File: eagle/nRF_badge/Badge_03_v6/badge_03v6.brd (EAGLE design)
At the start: 30 x 70 mm, 43 parts, among them U1 LIS2DH12", U2 LP2985LV, U3 MCP6231, U5 M95M02, Y1 32768Hz

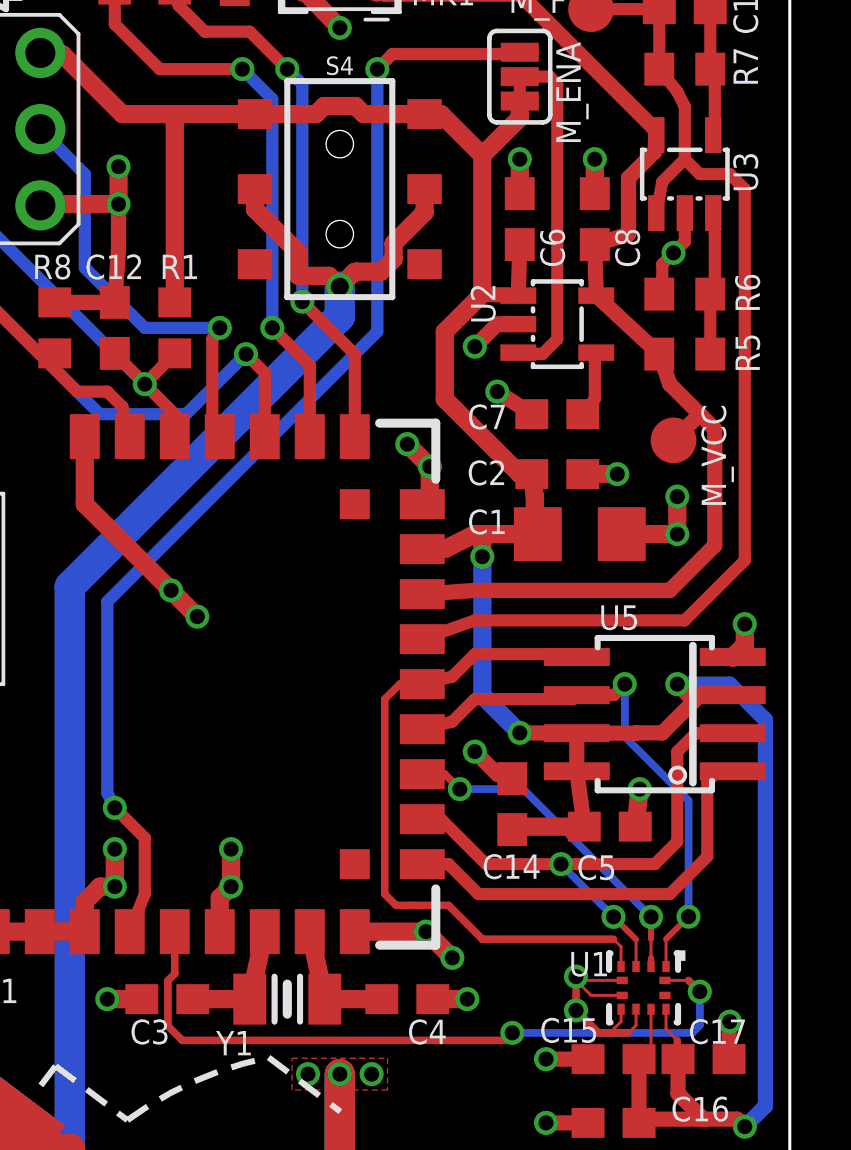
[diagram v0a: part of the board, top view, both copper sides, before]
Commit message: Updated DRC. Small fixed to board design
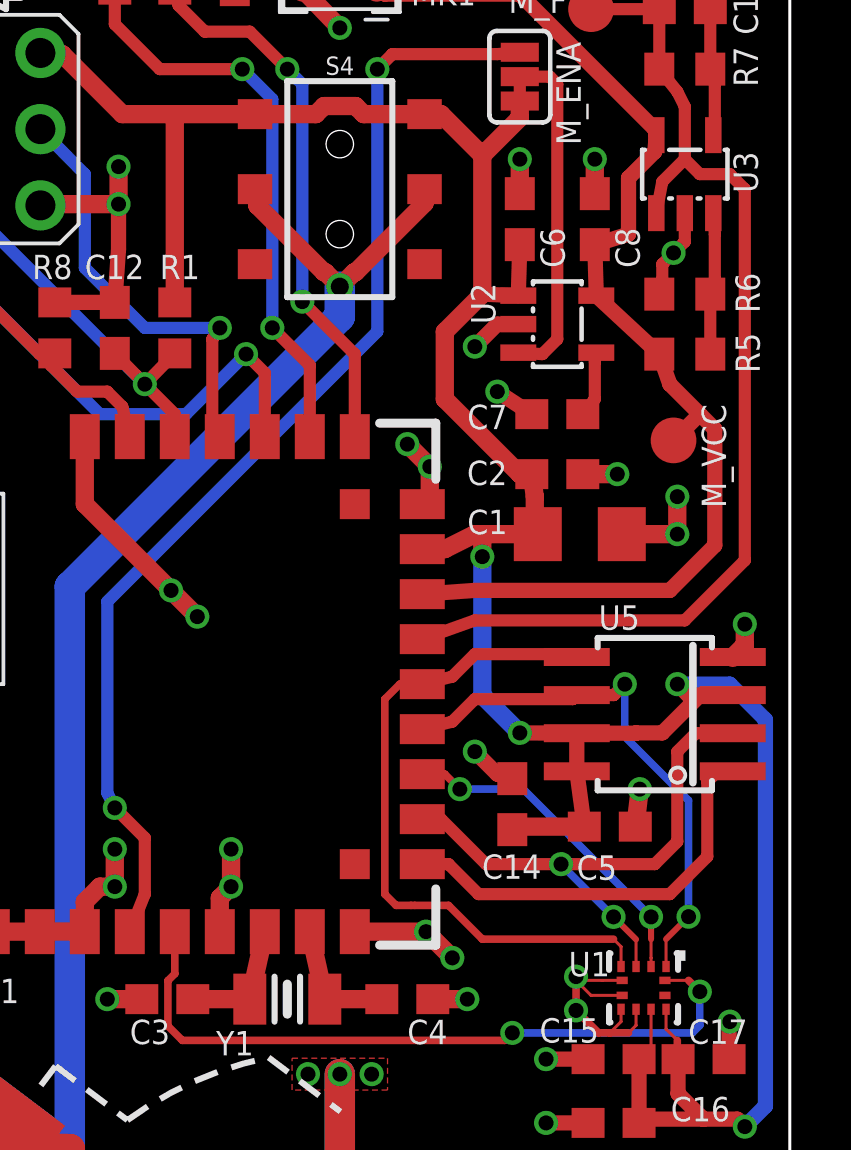
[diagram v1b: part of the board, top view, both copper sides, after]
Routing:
- net VBATT: track 140.7 -> 139.6 mm
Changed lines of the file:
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@@
 </class>
 </classes>
-<designrules name="PCBNG_DRC_by_oren *">
+<designrules name="PCBNG_DRC_by_oren">
 <description language="de">&lt;b&gt;EAGLE Design Rules&lt;/b&gt;
 &lt;p&gt;
@@
 <contactref element="S4" pad="5"/>
 <wire x1="12.25" y1="53" x2="12.175" y2="53" width="0.6096" layer="1"/>
-<wire x1="12.175" y1="53" x2="12.175" y2="52.325" width="0.6096" layer="1"/>
-<wire x1="13.625" y1="50.875" x2="13.625" y2="50.1096" width="0.6096" layer="1"/>
-<wire x1="12.175" y1="52.325" x2="13.625" y2="50.875" width="0.6096" layer="1"/>
-<wire x1="13.625" y1="50.1096" x2="14.6404" y2="50.1096" width="0.6096" layer="1"/>
-<wire x1="14.6404" y1="50.1096" x2="15" y2="49.75" width="0.6096" layer="1"/>
 <wire x1="15" y1="49.75" x2="15.48" y2="50.23" width="0.6096" layer="1"/>
 <wire x1="15.48" y1="50.23" x2="15.52605625" y2="50.23" width="0.6096" layer="1"/>
-<wire x1="15.52605625" y1="50.23" x2="15.54605625" y2="50.25" width="0.6096" layer="1"/>
-<wire x1="15.54605625" y1="50.25" x2="16.375" y2="50.25" width="0.6096" layer="1"/>
-<wire x1="16.375" y1="50.25" x2="16.7928" y2="50.6678" width="0.6096" layer="1"/>
-<wire x1="16.7928" y1="50.6678" x2="16.7928" y2="51.18938125" width="0.6096" layer="1"/>
-<wire x1="17.825" y1="52.22158125" x2="17.825" y2="53" width="0.6096" layer="1"/>
-<wire x1="16.7928" y1="51.18938125" x2="17.825" y2="52.22158125" width="0.6096" layer="1"/>
+<wire x1="15.52605625" y1="50.23" x2="17.825" y2="52.52894375" width="0.6096" layer="1"/>
+<wire x1="17.825" y1="52.52894375" x2="17.825" y2="53" width="0.6096" layer="1"/>
+<wire x1="15" y1="49.75" x2="14.52" y2="50.23" width="0.6096" layer="1"/>
+<wire x1="14.52" y1="50.23" x2="14.47394375" y2="50.23" width="0.6096" layer="1"/>
+<wire x1="14.47394375" y1="50.23" x2="12.25" y2="52.45394375" width="0.6096" layer="1"/>
+<wire x1="12.25" y1="52.45394375" x2="12.25" y2="53" width="0.6096" layer="1"/>
 </signal>
 <signal name="MOSI">
@@
 <wire x1="25.375" y1="28.742" x2="25.375" y2="28" width="0.2032" layer="1"/>
 <wire x1="25.375" y1="28" x2="25.375" y2="27.375" width="0.1016" layer="1"/>
-<wire x1="25.375" y1="27.375" x2="25.375" y2="27.0875" width="0.2032" layer="1"/>
+<wire x1="25.375" y1="27.375" x2="25.375" y2="27.0875" width="0.1016" layer="1"/>
 </signal>
 </signals>
